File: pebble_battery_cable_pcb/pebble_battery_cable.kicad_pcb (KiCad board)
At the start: 2 copper layers, 10.2 x 7.7 mm, 2 parts

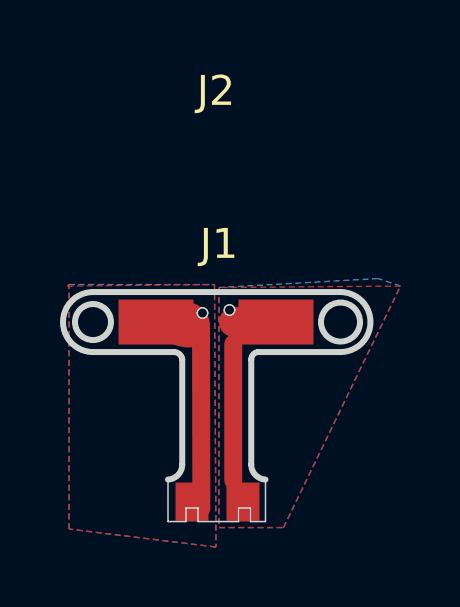
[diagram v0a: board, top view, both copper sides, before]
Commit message: sending off
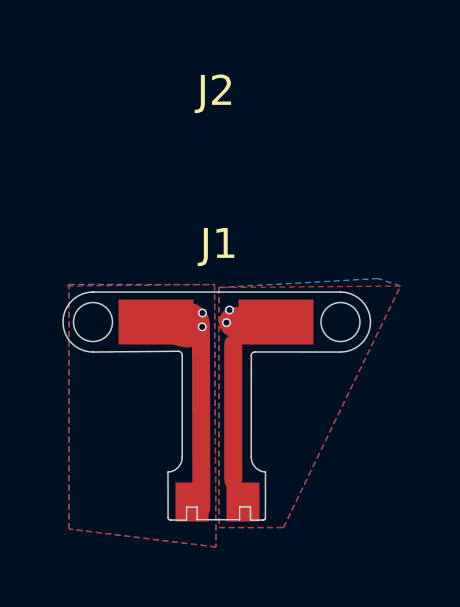
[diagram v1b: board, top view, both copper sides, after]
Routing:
- net VCC: track 0.58 -> 0.00 mm, vias 1 -> 2
- net GND: vias 1 -> 2
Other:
- board size 10.2 x 7.7 mm -> 10.2 x 7.6 mm
